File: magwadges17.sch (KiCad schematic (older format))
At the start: 23 parts, among them J1 CONN_02X03, J2 JACK_2P, Q1 BC846BDW1, Q2 BC846BDW1, U1 ATTINY2313-20MU, U2 FT25H16

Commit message: Updated schematic
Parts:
- removed D1, D2, D3, D4: LED, custom:LTST-C230KRKT, symbol LED
- removed Q1, Q2: BC846BDW1, TO_SOT_Packages_SMD:SOT-363_SC-70-6, symbol BC846BDW1
- removed R1, R2: 47, Resistors_SMD:R_0805, symbol R
- removed R3: 1K, Resistors_SMD:R_0805, symbol R
- removed R4, R5: 1M, Resistors_SMD:R_0805, symbol R
- removed R6, R7: 2K2, Resistors_SMD:R_0805, symbol R
- removed U1: ATTINY2313-20MU, Housings_DFN_QFN:QFN-20-1EP_4x4mm_Pitch0.5mm, symbol ATTINY2313-20MU
- removed U2: FT25H16, Housings_SOIC:SOIC-8_3.9x4.9mm_Pitch1.27mm, symbol FT25H16
- added RN1: R_Pack04, symbol R_Pack04
- added S5, S6, S7, S8: SW_SPST, custom:PTS645, symbol SW_SPST
- added U1: ATTINY861A-MU, QFN_MLF32, symbol ATTINY861A-MU
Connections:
- net labels added: SW_A, SW_B, SW_C, SW_D, SW_E, SW_F, SW_G, SW_H, TouchC
- wire segments 93 -> 66
- no-connect marks 8 -> 0
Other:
- moved on the sheet: J1, S1, S2, S3, S4

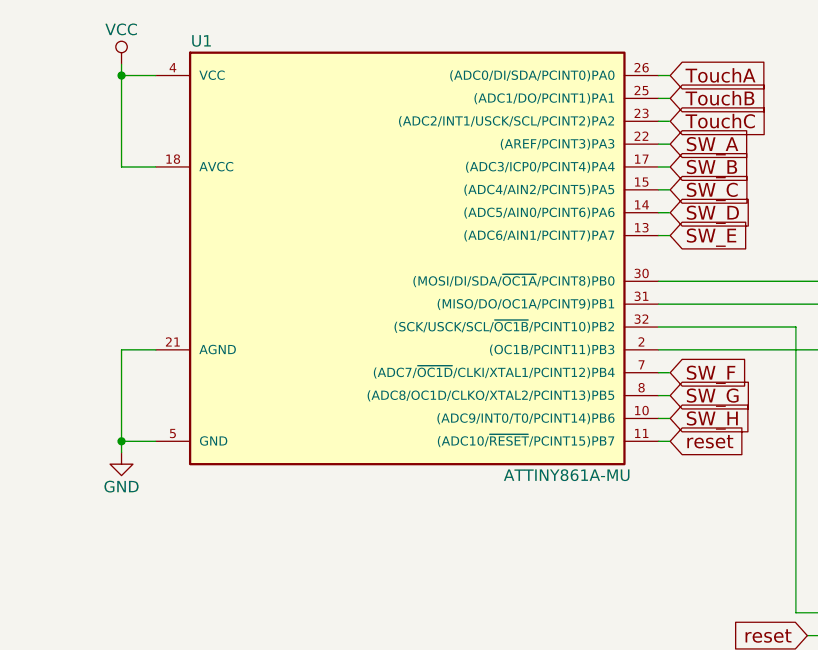
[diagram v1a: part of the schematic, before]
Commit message: Updated schematic
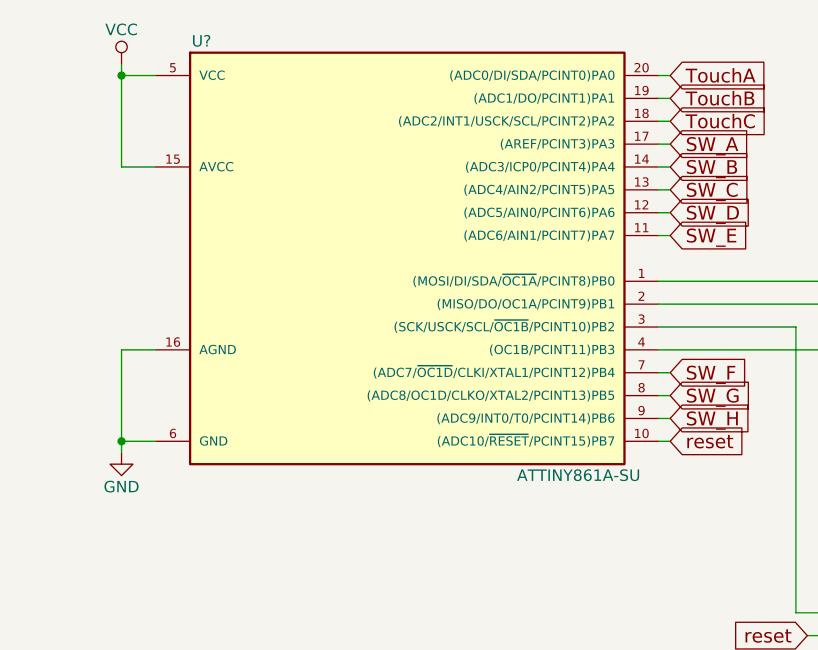
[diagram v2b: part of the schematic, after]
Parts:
- removed U1: ATTINY861A-MU, QFN_MLF32, symbol ATTINY861A-MU
- added U?: ATTINY861A-SU, Housings_SOIC:SOIC-20W_7.5x12.8mm_Pitch1.27mm, symbol ATTINY861A-SU
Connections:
- net GND: now also U?.16 (AGND), U?.6 (GND)
- net SW_A: now also U?.17 ((AREF/PCINT3)PA3)
- net SW_B: now also U?.14 ((ADC3/ICP0/PCINT4)PA4)
- net SW_C: now also U?.13 ((ADC4/AIN2/PCINT5)PA5)
- net SW_D: now also U?.12 ((ADC5/AIN0/PCINT6)PA6)
- net SW_E: now also U?.11 ((ADC6/AIN1/PCINT7)PA7)
- net SW_F: now also U?.7 ((ADC7/~OC1D~/CLKI/XTAL1/PCINT12)PB4)
- net SW_G: now also U?.8 ((ADC8/OC1D/CLKO/XTAL2/PCINT13)PB5)
- net SW_H: now also U?.9 ((ADC9/INT0/T0/PCINT14)PB6)
- net TouchA: now also U?.20 ((ADC0/DI/SDA/PCINT0)PA0)
- net TouchB: now also U?.19 ((ADC1/DO/PCINT1)PA1)
- net TouchC: now also U?.18 ((ADC2/INT1/USCK/SCL/PCINT2)PA2)
- net VCC: now also U?.15 (AVCC), U?.5 (VCC)
- net reset: now also U?.10 ((ADC10/~RESET~/PCINT15)PB7)
- net at J2.2, J2.3, LS1.1: now also U?.4 ((OC1B/PCINT11)PB3)
- net at J1.1 (P1): now also U?.2 ((MISO/DO/OC1A/PCINT9)PB1)
- net at J1.3 (P3): now also U?.3 ((SCK/USCK/SCL/~OC1B~/PCINT10)PB2)
- net at J1.4 (P4): now also U?.1 ((MOSI/DI/SDA/~OC1A~/PCINT8)PB0)
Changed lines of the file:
@@
 Wire Wire Line
 	7750 5250 7750 5200
-$Comp
-L ATTINY861A-MU U1
-U 1 1 597BCA60
-P 4050 2050
-F 0 "U1" H 3150 3000 50  0000 C CNN
-F 1 "ATTINY861A-MU" H 4750 1100 50  0000 C CNN
-F 2 "QFN_MLF32" H 4050 2050 50  0001 C CIN
-F 3 "" H 4050 2050 50  0001 C CNN
-	1    4050 2050
-	1    0    0    -1
-$EndComp
 Wire Wire Line
 	6400 3500 6350 3500
@@
 Wire Wire Line
 	7250 2050 7900 2050
+$Comp
+L ATTINY861A-SU U?
+U 1 1 597BFFA6
+P 4050 2050
+F 0 "U?" H 3150 3000 50  0000 C CNN
+F 1 "ATTINY861A-SU" H 4800 1100 50  0000 C CNN
+F 2 "Housings_SOIC:SOIC-20W_7.5x12.8mm_Pitch1.27mm" H 4050 2050 50  0001 C CIN
+F 3 "" H 4050 2050 50  0001 C CNN
+	1    4050 2050
+	1    0    0    -1
+$EndComp
 $EndSCHEMATC
